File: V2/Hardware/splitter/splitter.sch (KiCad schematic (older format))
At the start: 21 parts, among them J0 Rpi_40Pin_F, J1 Control_seg:1, J2 Control_seg:2, J3 Control_seg:3, J4 Molex_PSU_F, J5 Siren, J6 USB_A_F, K0 RELRAS0515, Q1 BD139-16

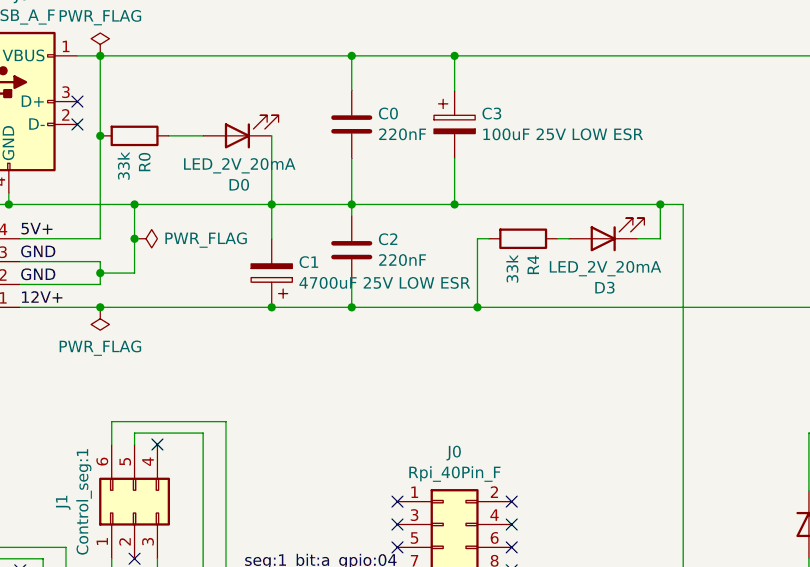
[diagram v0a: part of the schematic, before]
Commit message: Update files
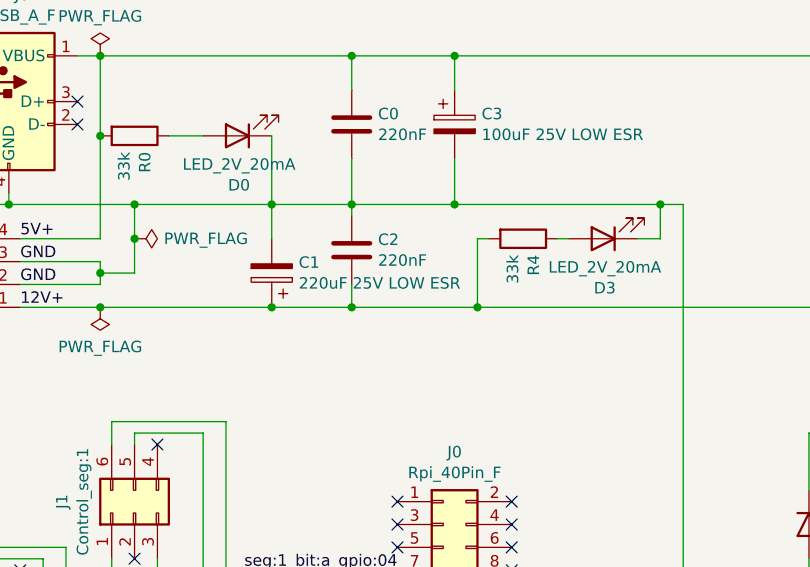
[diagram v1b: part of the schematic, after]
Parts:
- C1: value 4700uF 25V LOW ESR -> 220uF 25V LOW ESR; footprint Capacitor_THT:CP_Radial_D18.0mm_P7.50mm -> Capacitor_THT:CP_Radial_D8.0mm_P3.50mm
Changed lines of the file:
@@
 P 5050 2700
 F 0 "C1" H 4932 2654 50  0000 R CNN
-F 1 "4700uF 25V LOW ESR" H 4932 2745 50  0000 R CNN
-F 2 "Capacitor_THT:CP_Radial_D18.0mm_P7.50mm" H 5088 2550 50  0001 C CNN
+F 1 "220uF 25V LOW ESR" H 4932 2745 50  0000 R CNN
+F 2 "Capacitor_THT:CP_Radial_D8.0mm_P3.50mm" H 5088 2550 50  0001 C CNN
 F 3 "~" H 5050 2700 50  0001 C CNN
 	1    5050 2700
